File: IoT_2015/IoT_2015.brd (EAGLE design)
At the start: 100 x 80 mm, 29 parts, among them Y1 ABLS-16.000MHZ-B4-T

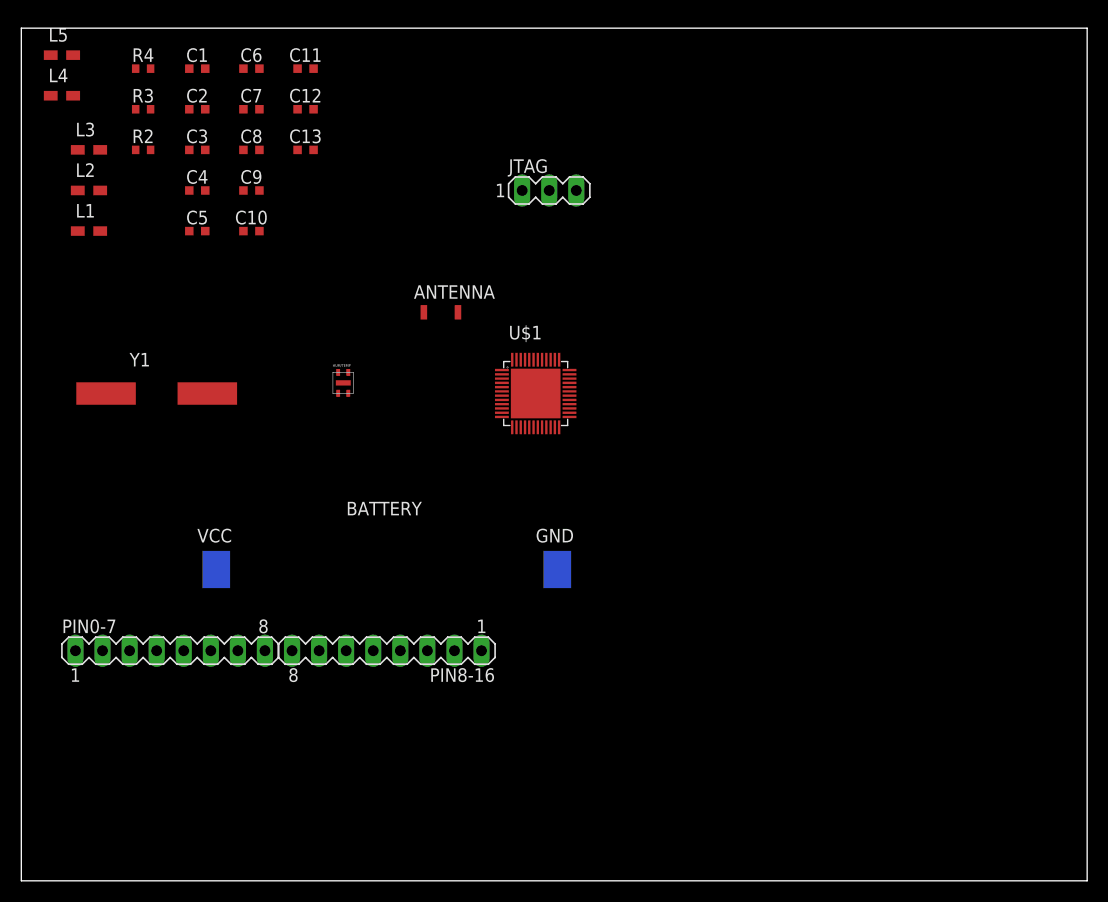
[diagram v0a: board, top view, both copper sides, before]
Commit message: First board design finished
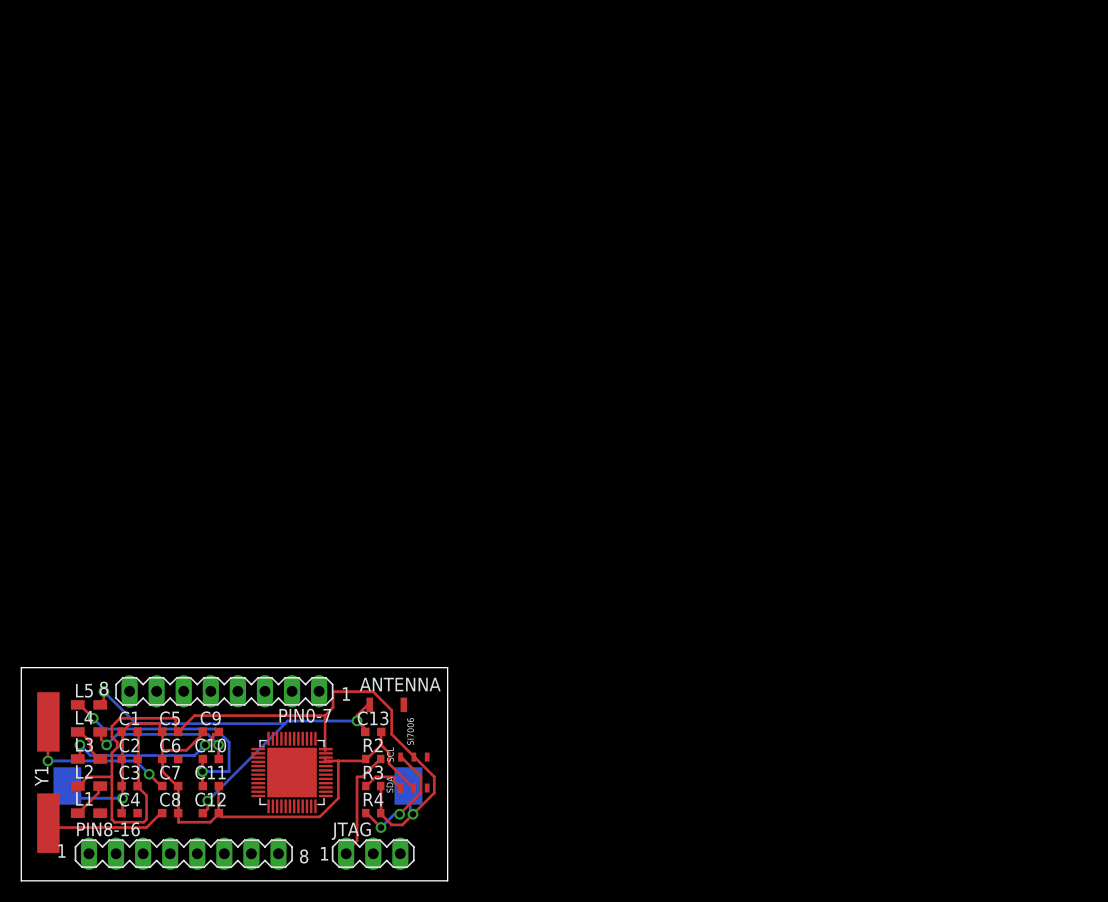
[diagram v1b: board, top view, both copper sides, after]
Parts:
- removed HUM/TEMP: SHTC1, Sensirion:4INPUTS
- added SI7006: SI7006-A20-IM, SiliconLabs:SI7006-A20-IM
- moved R4 73.1 mm to (33.0, 6.35)
- moved C11 67.9 mm to (17.8, 8.89)
- moved R3 67.1 mm to (33.0, 8.89)
- moved C12 66.6 mm to (17.8, 6.35)
- moved C6 65.2 mm to (14.0, 11.4)
- moved JTAG 64.4 mm to (33.0, 2.54)
- moved C7 64.0 mm to (14.0, 8.89)
- moved C8 62.7 mm to (14.0, 6.35)
- moved C1 62.6 mm to (10.2, 14.0)
- moved C2 61.3 mm to (10.2, 11.4)
- moved R2 61.1 mm to (33.0, 11.4)
- moved L5 61.0 mm to (6.35, 16.5)
- moved C3 60.0 mm to (10.2, 8.89)
- moved L4 59.7 mm to (6.35, 14.0)
- moved C4 58.8 mm to (10.2, 6.35)
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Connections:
- net GND: now also SI7006.GND; no longer HUM/TEMP.VSS
- net SCL: now also SI7006.SCL; no longer HUM/TEMP.SCL
- net SDA: now also SI7006.SDA; no longer HUM/TEMP.SDA
- net VDD: now also SI7006.VDD; no longer HUM/TEMP.VDD
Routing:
- net VDD: track 0.00 -> 80.9 mm, vias 0 -> 1
- net GND: track 0.00 -> 67.3 mm, vias 0 -> 1
- net N$4: track 0.00 -> 41.5 mm, vias 0 -> 3
- net N$11: track 0.00 -> 23.4 mm, vias 0 -> 2
- net N$5: track 0.00 -> 16.1 mm, vias 0 -> 2
- net N$10: track 0.00 -> 15.3 mm, vias 0 -> 2
- net N$7: track 0.00 -> 14.1 mm, vias 0 -> 2
- net N$9: track 0.00 -> 11.5 mm
- net SCL: track 0.00 -> 11.2 mm, vias 0 -> 2
- net SWDCLK: track 0.00 -> 10.5 mm
- net SDA: track 0.00 -> 4.32 mm
- net N$6: track 0.00 -> 3.59 mm
- net N$1: track 0.00 -> 3.43 mm
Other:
- board size 100 x 80 mm -> 40 x 20 mm
- board text added: "BlueNinc"
